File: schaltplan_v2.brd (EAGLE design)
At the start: 100 x 80 mm, 43 parts, among them T1 2N3565, T2 2N3565, T3 2N3565, T4 2N3565, T5 2N3565, T6 2N3565, T7 2N3565, T8 2N3565

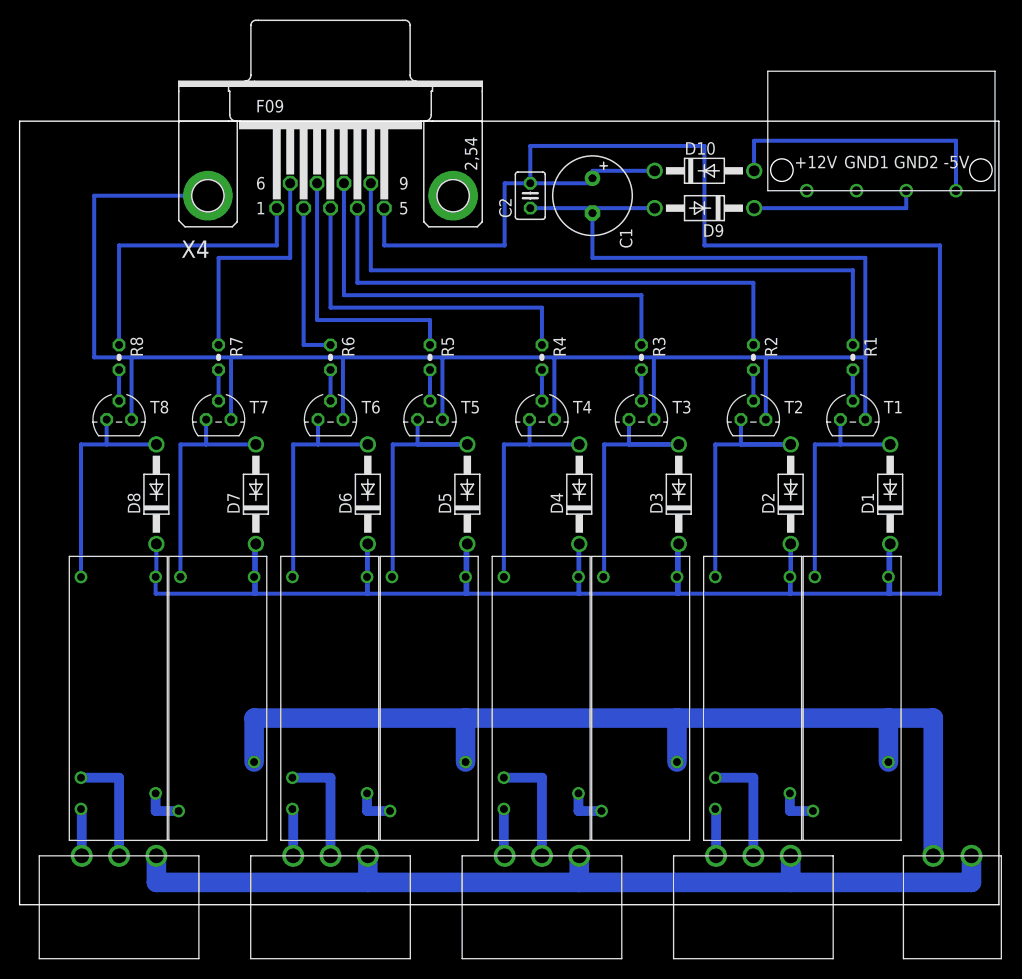
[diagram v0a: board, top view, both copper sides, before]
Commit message: more layout fixes
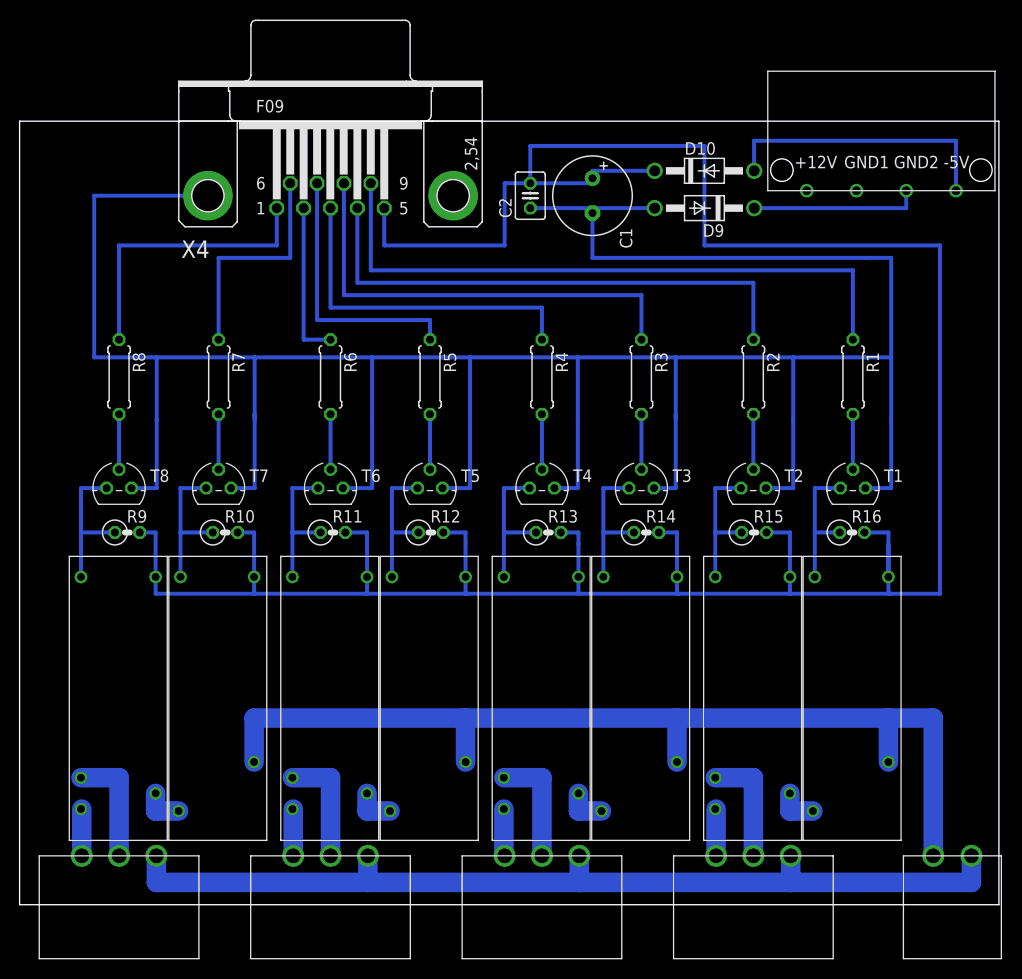
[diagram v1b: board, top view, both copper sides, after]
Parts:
- removed D1, D2, D3, D4, D5, D6, D7, D8: 1N4004, diode:DO41-10
- added R10, R11, R12, R13, R14, R15, R16, R9: (no value), rcl:0207/2V
- R1, R2, R3, R4, R5, R6, R7, R8: device resistor:0204V -> rcl:0207/7
- moved T1 7.00 mm to (85.1, 42.5)
- moved T2 7.00 mm to (74.9, 42.5)
- moved T3 7.00 mm to (63.5, 42.5)
- moved T4 7.00 mm to (53.3, 42.5)
- moved T5 7.00 mm to (41.9, 42.5)
- moved T6 7.00 mm to (31.8, 42.5)
- moved T7 7.00 mm to (20.3, 42.5)
- moved T8 7.00 mm to (10.2, 42.5)
- moved R1 2.00 mm to (85.1, 53.9)
- moved R2 2.00 mm to (74.9, 53.9)
- moved R3 2.00 mm to (63.5, 53.9)
- moved R4 2.00 mm to (53.3, 53.9)
- moved R5 2.00 mm to (41.9, 53.9)
- moved R6 2.00 mm to (31.8, 53.9)
- moved R7 2.00 mm to (20.3, 53.9)
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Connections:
- new net N$10: X4.G2
- net N$12: now also R15.1; no longer D2.A
- net N$20: now also R14.1; no longer D3.A
- net N$24: now also R10.2, R11.2, R12.2, R13.2, R14.2, R15.2, R16.2, R9.2; no longer D1.C, D2.C, D3.C, D4.C, D5.C, D6.C, D7.C, D8.C
- net N$25: now also R13.1; no longer D4.A
- net N$34: now also R12.1; no longer D5.A
- net N$39: now also R11.1; no longer D6.A
- net N$46: now also R10.1; no longer D7.A
- net N$51: now also R9.1; no longer D8.A
- net N$6: now also R16.1; no longer D1.A
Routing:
- net N$19: track 213.5 -> 296.6 mm
- net N$12: track 28.8 -> 14.4 mm
- net N$34: track 28.8 -> 14.4 mm
- net N$20: track 28.9 -> 14.8 mm
- net N$6: track 23.8 -> 14.2 mm
- net N$39: track 23.8 -> 14.6 mm
- net N$25: track 23.8 -> 15.0 mm
- net N$46: track 23.8 -> 15.0 mm
- net N$51: track 23.8 -> 15.2 mm
- net N$24: track 287.7 -> 279.8 mm
- net N$8: track 3.17 -> 5.63 mm
- net N$48: track 3.17 -> 5.63 mm
- net N$40: track 3.17 -> 5.63 mm
- net N$36: track 3.17 -> 5.63 mm
- net N$28: track 3.17 -> 5.63 mm
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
